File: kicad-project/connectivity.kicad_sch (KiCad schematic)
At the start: 21 parts, among them J5 Conn_01x04, Q1 3LP01M, Q2 PDTC114Y, Q3 Q_NPN_BCE, U4 PAM-7Q-0

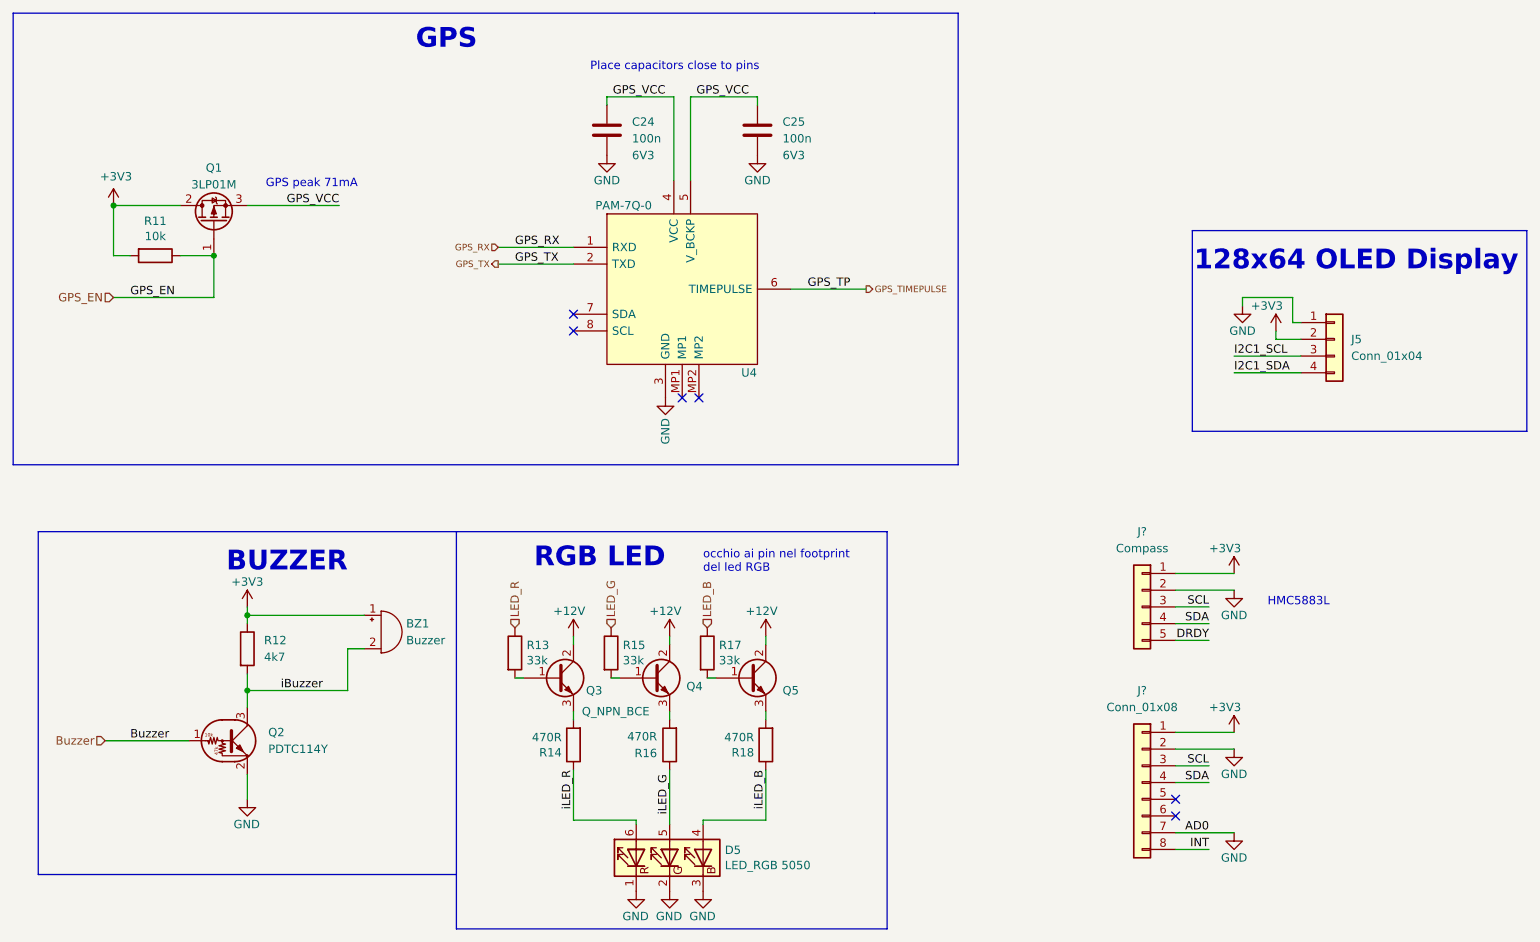
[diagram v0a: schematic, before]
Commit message: commit anonimo di thimas
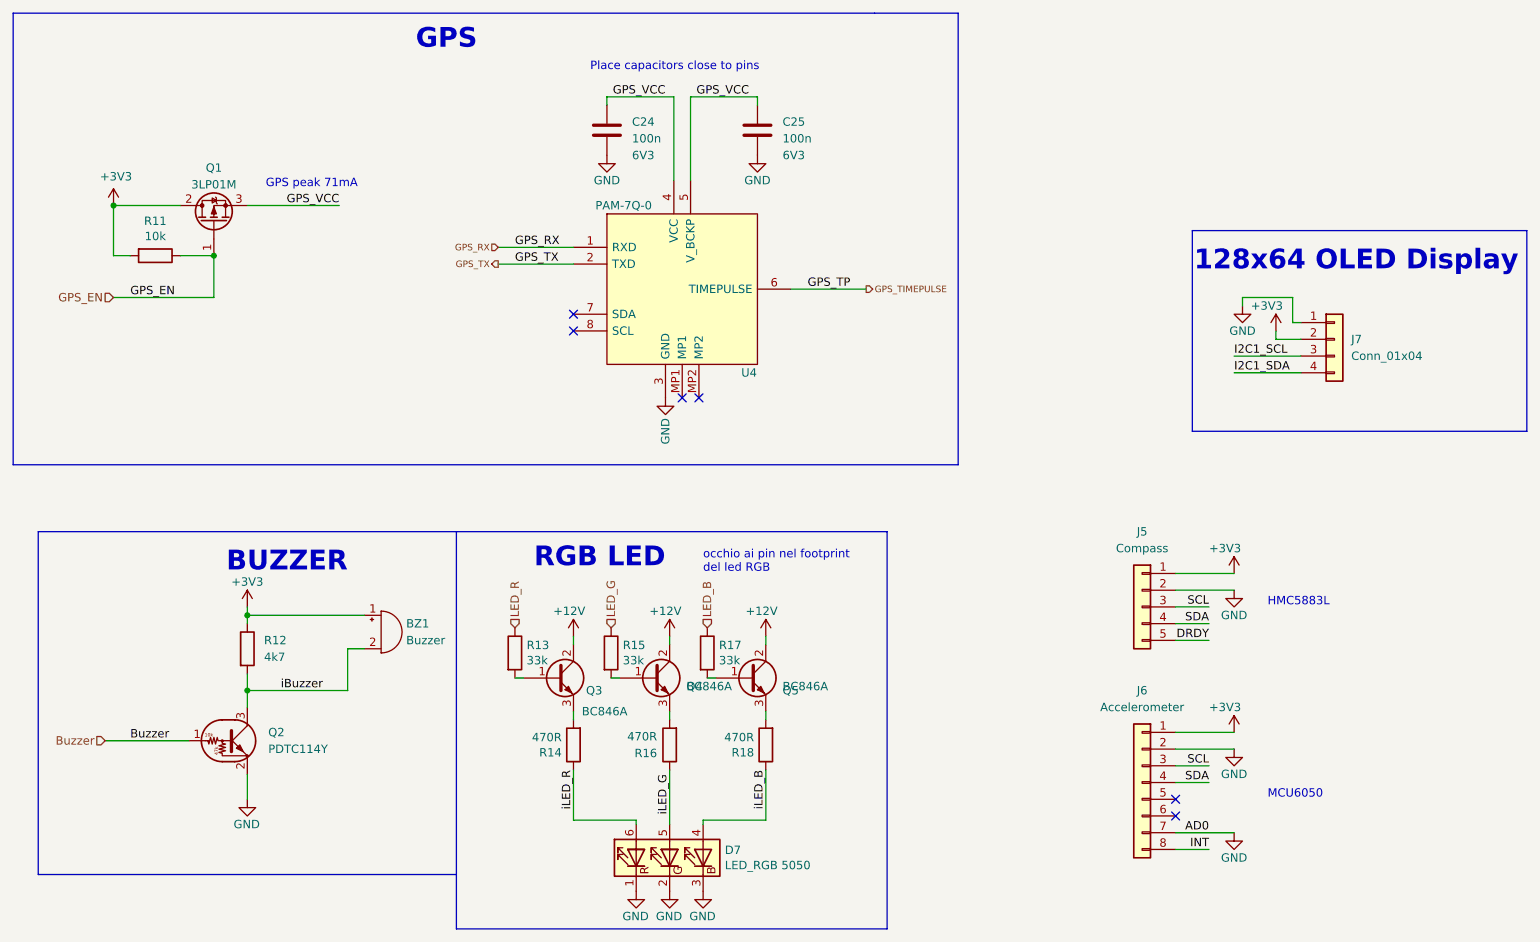
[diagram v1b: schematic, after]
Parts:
- J6: renamed from J?; value Conn_01x08 -> Accelerometer
- Q2: footprint (none) -> Package_TO_SOT_SMD:SOT-23
- Q3: value Q_NPN_BCE -> BC846A; footprint (none) -> Package_TO_SOT_SMD:SOT-23
- Q4, Q5: value ~ -> BC846A; footprint (none) -> Package_TO_SOT_SMD:SOT-23
- gave numbers to parts that had none: 1
- renumbered D5 to D7, J5 to J7
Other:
- note added: "MCU6050"
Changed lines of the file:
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@@
     (stroke (width 0) (type default) (color 0 0 0 0))
+  )
+  (text "MCU6050" (at 204.47 133.35 0)
+    (effects (font (size 1.27 1.27)) (justify left bottom))
   )
   (text "RGB LED" (at 113.03 98.425 180)
@@
   (symbol (lib_id "power:+3V3") (at 29.21 43.18 0) (unit 1)
     (in_bom yes) (on_board yes)
-    (property "Reference" "#PWR054" (id 0) (at 29.21 46.99 0)
+    (property "Reference" "#PWR057" (id 0) (at 29.21 46.99 0)
       (effects (font (size 1.27 1.27)) hide)
     )
@@
   (symbol (lib_id "power:GND") (at 113.03 72.39 0) (unit 1)
     (in_bom yes) (on_board yes)
-    (property "Reference" "#PWR060" (id 0) (at 113.03 78.74 0)
+    (property "Reference" "#PWR063" (id 0) (at 113.03 78.74 0)
       (effects (font (size 1.27 1.27)) hide)
     )
@@
   (symbol (lib_id "power:GND") (at 199.39 101.6 0) (unit 1)
     (in_bom yes) (on_board yes)
-    (property "Reference" "#PWR?" (id 0) (at 199.39 107.95 0)
+    (property "Reference" "#PWR070" (id 0) (at 199.39 107.95 0)
       (effects (font (size 1.27 1.27)) hide)
     )
@@
   (symbol (lib_id "power:GND") (at 104.14 35.56 0) (unit 1)
     (in_bom yes) (on_board yes)
-    (property "Reference" "#PWR058" (id 0) (at 104.14 41.91 0)
+    (property "Reference" "#PWR061" (id 0) (at 104.14 41.91 0)
       (effects (font (size 1.27 1.27)) hide)
     )
@@
   (symbol (lib_id "power:+3V3") (at 49.53 104.14 0) (unit 1)
     (in_bom yes) (on_board yes)
-    (property "Reference" "#PWR055" (id 0) (at 49.53 107.95 0)
+    (property "Reference" "#PWR058" (id 0) (at 49.53 107.95 0)
       (effects (font (size 1.27 1.27)) hide)
     )
@@
   (symbol (lib_id "power:GND") (at 108.585 147.32 0) (unit 1)
     (in_bom yes) (on_board yes)
-    (property "Reference" "#PWR059" (id 0) (at 108.585 153.67 0)
+    (property "Reference" "#PWR062" (id 0) (at 108.585 153.67 0)
       (effects (font (size 1.27 1.27)) hide)
     )
@@
   (symbol (lib_id "Connector_Generic:Conn_01x04") (at 214.63 63.5 0) (unit 1)
     (in_bom yes) (on_board yes) (fields_autoplaced)
-    (property "Reference" "J5" (id 0) (at 217.17 63.4999 0)
+    (property "Reference" "J7" (id 0) (at 217.17 63.4999 0)
       (effects (font (size 1.27 1.27)) (justify left))
     )
@@
       (effects (font (size 1.27 1.27)) (justify left))
     )
-    (property "Value" "~" (id 1) (at 116.205 116.2049 0)
-      (effects (font (size 1.27 1.27)) (justify left))
-    )
-    (property "Footprint" "" (id 2) (at 116.205 112.395 0)
-      (effects (font (size 1.27 1.27)) hide)
-    )
-    (property "Datasheet" "~" (id 3) (at 111.125 114.935 0)
+    (property "Value" "BC846A" (id 1) (at 116.205 116.2049 0)
+      (effects (font (size 1.27 1.27)) (justify left))
+    )
+    (property "Footprint" "Package_TO_SOT_SMD:SOT-23" (id 2) (at 116.205 112.395 0)
+      (effects (font (size 1.27 1.27)) hide)
+    )
+    (property "Datasheet" "https://www.mouser.it/datasheet/2/308/1/BC846ALT1_D-2310268.pdf" (id 3) (at 111.125 114.935 0)
       (effects (font (size 1.27 1.27)) hide)
     )
@@
   (symbol (lib_id "power:GND") (at 199.39 138.43 0) (unit 1)
     (in_bom yes) (on_board yes)
-    (property "Reference" "#PWR?" (id 0) (at 199.39 144.78 0)
+    (property "Reference" "#PWR073" (id 0) (at 199.39 144.78 0)
       (effects (font (size 1.27 1.27)) hide)
     )
@@
   (symbol (lib_id "power:+3V3") (at 205.74 62.23 0) (unit 1)
     (in_bom yes) (on_board yes)
-    (property "Reference" "#PWR067" (id 0) (at 205.74 66.04 0)
+    (property "Reference" "#PWR075" (id 0) (at 205.74 66.04 0)
       (effects (font (size 1.27 1.27)) hide)
     )
@@
   (symbol (lib_id "power:GND") (at 113.665 147.32 0) (unit 1)
     (in_bom yes) (on_board yes)
-    (property "Reference" "#PWR062" (id 0) (at 113.665 153.67 0)
+    (property "Reference" "#PWR065" (id 0) (at 113.665 153.67 0)
       (effects (font (size 1.27 1.27)) hide)
     )
@@
   (symbol (lib_id "power:+12V") (at 128.27 108.585 0) (unit 1)
     (in_bom yes) (on_board yes)
-    (property "Reference" "#PWR065" (id 0) (at 128.27 112.395 0)
+    (property "Reference" "#PWR068" (id 0) (at 128.27 112.395 0)
       (effects (font (size 1.27 1.27)) hide)
     )
@@
   (symbol (lib_id "power:+3V3") (at 199.39 123.19 0) (unit 1)
     (in_bom yes) (on_board yes)
-    (property "Reference" "#PWR?" (id 0) (at 199.39 127 0)
+    (property "Reference" "#PWR071" (id 0) (at 199.39 127 0)
       (effects (font (size 1.27 1.27)) hide)
     )
@@
   (symbol (lib_id "power:+12V") (at 99.06 108.585 0) (unit 1)
     (in_bom yes) (on_board yes)
-    (property "Reference" "#PWR057" (id 0) (at 99.06 112.395 0)
+    (property "Reference" "#PWR060" (id 0) (at 99.06 112.395 0)
       (effects (font (size 1.27 1.27)) hide)
     )
@@
   (symbol (lib_id "power:+12V") (at 113.665 108.585 0) (unit 1)
     (in_bom yes) (on_board yes)
-    (property "Reference" "#PWR061" (id 0) (at 113.665 112.395 0)
+    (property "Reference" "#PWR064" (id 0) (at 113.665 112.395 0)
       (effects (font (size 1.27 1.27)) hide)
     )
@@
   (symbol (lib_id "power:+3V3") (at 199.39 99.06 0) (unit 1)
     (in_bom yes) (on_board yes)
-    (property "Reference" "#PWR?" (id 0) (at 199.39 102.87 0)
+    (property "Reference" "#PWR069" (id 0) (at 199.39 102.87 0)
       (effects (font (size 1.27 1.27)) hide)
     )
@@
   (symbol (lib_id "power:GND") (at 118.745 147.32 0) (unit 1)
     (in_bom yes) (on_board yes)
-    (property "Reference" "#PWR063" (id 0) (at 118.745 153.67 0)
+    (property "Reference" "#PWR066" (id 0) (at 118.745 153.67 0)
       (effects (font (size 1.27 1.27)) hide)
     )
@@
   (symbol (lib_id "power:GND") (at 200.66 58.42 0) (unit 1)
     (in_bom yes) (on_board yes)
-    (property "Reference" "#PWR066" (id 0) (at 200.66 64.77 0)
+    (property "Reference" "#PWR074" (id 0) (at 200.66 64.77 0)
       (effects (font (size 1.27 1.27)) hide)
     )
@@
   (symbol (lib_id "power:GND") (at 127 35.56 0) (unit 1)
     (in_bom yes) (on_board yes)
-    (property "Reference" "#PWR064" (id 0) (at 127 41.91 0)
+    (property "Reference" "#PWR067" (id 0) (at 127 41.91 0)
       (effects (font (size 1.27 1.27)) hide)
     )
@@
   (symbol (lib_id "Connector_Generic:Conn_01x05") (at 185.42 104.14 0) (mirror y) (unit 1)
     (in_bom yes) (on_board yes) (fields_autoplaced)
-    (property "Reference" "J?" (id 0) (at 185.42 92.71 0))
+    (property "Reference" "J5" (id 0) (at 185.42 92.71 0))
     (property "Value" "Compass" (id 1) (at 185.42 95.25 0))
     (property "Footprint" "" (id 2) (at 185.42 104.14 0)
@@
   (symbol (lib_id "Connector_Generic:Conn_01x08") (at 185.42 130.81 0) (mirror y) (unit 1)
     (in_bom yes) (on_board yes) (fields_autoplaced)
-    (property "Reference" "J?" (id 0) (at 185.42 116.84 0))
-    (property "Value" "Conn_01x08" (id 1) (at 185.42 119.38 0))
+    (property "Reference" "J6" (id 0) (at 185.42 116.84 0))
+    (property "Value" "Accelerometer" (id 1) (at 185.42 119.38 0))
     (property "Footprint" "" (id 2) (at 185.42 130.81 0)
       (effects (font (size 1.27 1.27)) hide)
@@
   (symbol (lib_id "power:GND") (at 49.53 133.35 0) (unit 1)
     (in_bom yes) (on_board yes)
-    (property "Reference" "#PWR056" (id 0) (at 49.53 139.7 0)
+    (property "Reference" "#PWR059" (id 0) (at 49.53 139.7 0)
       (effects (font (size 1.27 1.27)) hide)
     )
@@
       (effects (font (size 1.27 1.27)) (justify left))
     )
-    (property "Value" "Q_NPN_BCE" (id 1) (at 100.33 120.015 0)
-      (effects (font (size 1.27 1.27)) (justify left))
-    )
-    (property "Footprint" "" (id 2) (at 101.6 112.395 0)
-      (effects (font (size 1.27 1.27)) hide)
-    )
-    (property "Datasheet" "~" (id 3) (at 96.52 114.935 0)
+    (property "Value" "BC846A" (id 1) (at 100.33 120.015 0)
+      (effects (font (size 1.27 1.27)) (justify left))
+    )
+    (property "Footprint" "Package_TO_SOT_SMD:SOT-23" (id 2) (at 101.6 112.395 0)
+      (effects (font (size 1.27 1.27)) hide)
+    )
+    (property "Datasheet" "https://www.mouser.it/datasheet/2/308/1/BC846ALT1_D-2310268.pdf" (id 3) (at 96.52 114.935 0)
       (effects (font (size 1.27 1.27)) hide)
     )
@@
       (effects (font (size 1.27 1.27)) (justify left))
     )
-    (property "Value" "~" (id 1) (at 130.81 116.2049 0)
-      (effects (font (size 1.27 1.27)) (justify left))
-    )
-    (property "Footprint" "" (id 2) (at 130.81 112.395 0)
-      (effects (font (size 1.27 1.27)) hide)
-    )
-    (property "Datasheet" "~" (id 3) (at 125.73 114.935 0)
+    (property "Value" "BC846A" (id 1) (at 130.81 116.2049 0)
+      (effects (font (size 1.27 1.27)) (justify left))
+    )
+    (property "Footprint" "Package_TO_SOT_SMD:SOT-23" (id 2) (at 130.81 112.395 0)
+      (effects (font (size 1.27 1.27)) hide)
+    )
+    (property "Datasheet" "https://www.mouser.it/datasheet/2/308/1/BC846ALT1_D-2310268.pdf" (id 3) (at 125.73 114.935 0)
       (effects (font (size 1.27 1.27)) hide)
     )
@@
   (symbol (lib_id "power:GND") (at 199.39 125.73 0) (unit 1)
     (in_bom yes) (on_board yes)
-    (property "Reference" "#PWR?" (id 0) (at 199.39 132.08 0)
+    (property "Reference" "#PWR072" (id 0) (at 199.39 132.08 0)
       (effects (font (size 1.27 1.27)) hide)
     )
@@
   (symbol (lib_id "Device:LED_RGB") (at 113.665 142.24 90) (unit 1)
     (in_bom yes) (on_board yes)
-    (property "Reference" "D5" (id 0) (at 122.047 141.0716 90)
+    (property "Reference" "D7" (id 0) (at 122.047 141.0716 90)
       (effects (font (size 1.27 1.27)) (justify right))
     )
@@
       (effects (font (size 1.27 1.27)) (justify left))
     )
-    (property "Footprint" "" (id 2) (at 46.99 124.46 0)
-      (effects (font (size 1.27 1.27)) (justify left) hide)
-    )
+    (property "Footprint" "Package_TO_SOT_SMD:SOT-23" (id 2) (at 46.99 124.46 0)
+      (effects (font (size 1.27 1.27)) (justify left) hide)
+    )
